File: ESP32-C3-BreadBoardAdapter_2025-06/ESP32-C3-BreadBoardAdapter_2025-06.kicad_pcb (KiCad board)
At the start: 2 copper layers, 52.1 x 40.6 mm, 32 parts, among them J1 PWR, J2 USB-C_Receptacle_Data_16P_GCT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, J3 PWR_JMP, J4 PWR_JMP, J6 Debug_3V3, SW1 SW_Push_SMD_6x3.5, SW2 SW_Push_SMD_6x3.5, SW3 SW_Push_SMD_6x3.5, U1 ESP32-C3-WROOM-02-N4, U2 AMS1117-3V3, U3 L7805

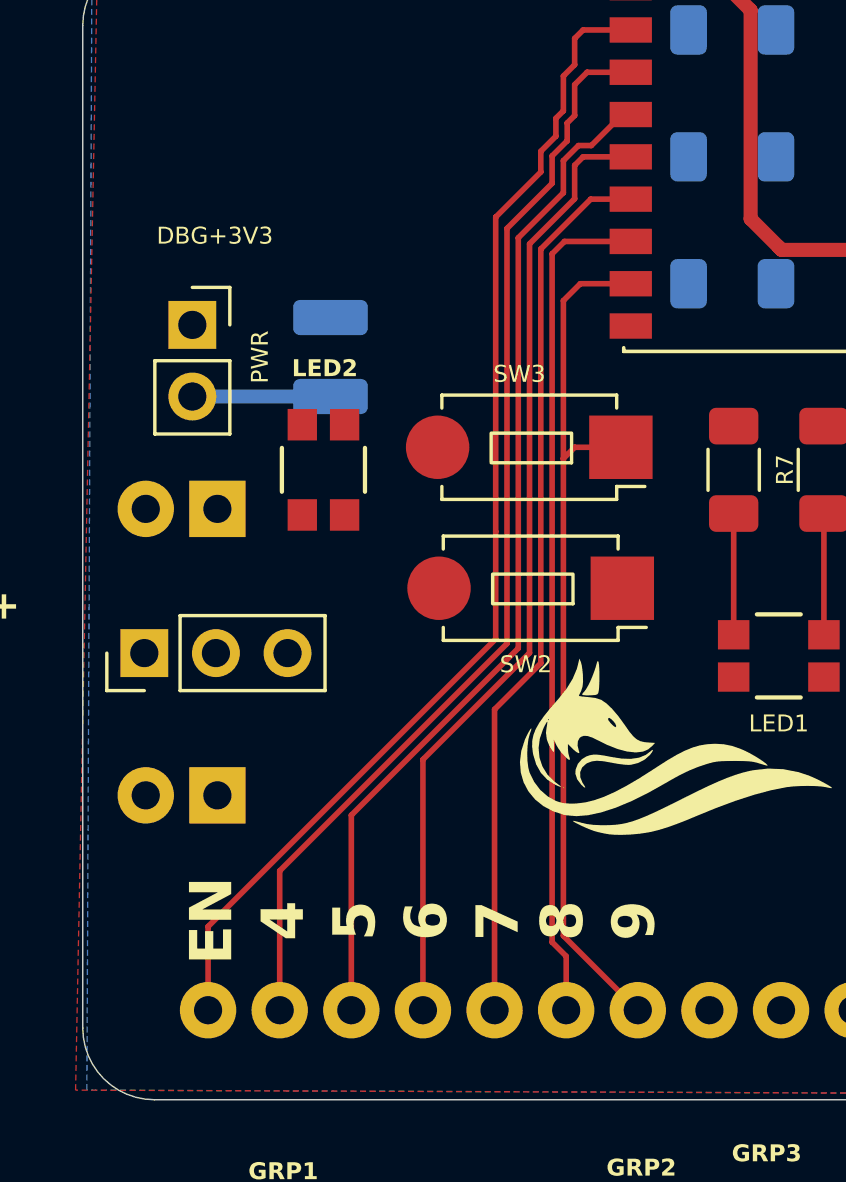
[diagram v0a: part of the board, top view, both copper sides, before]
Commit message: .
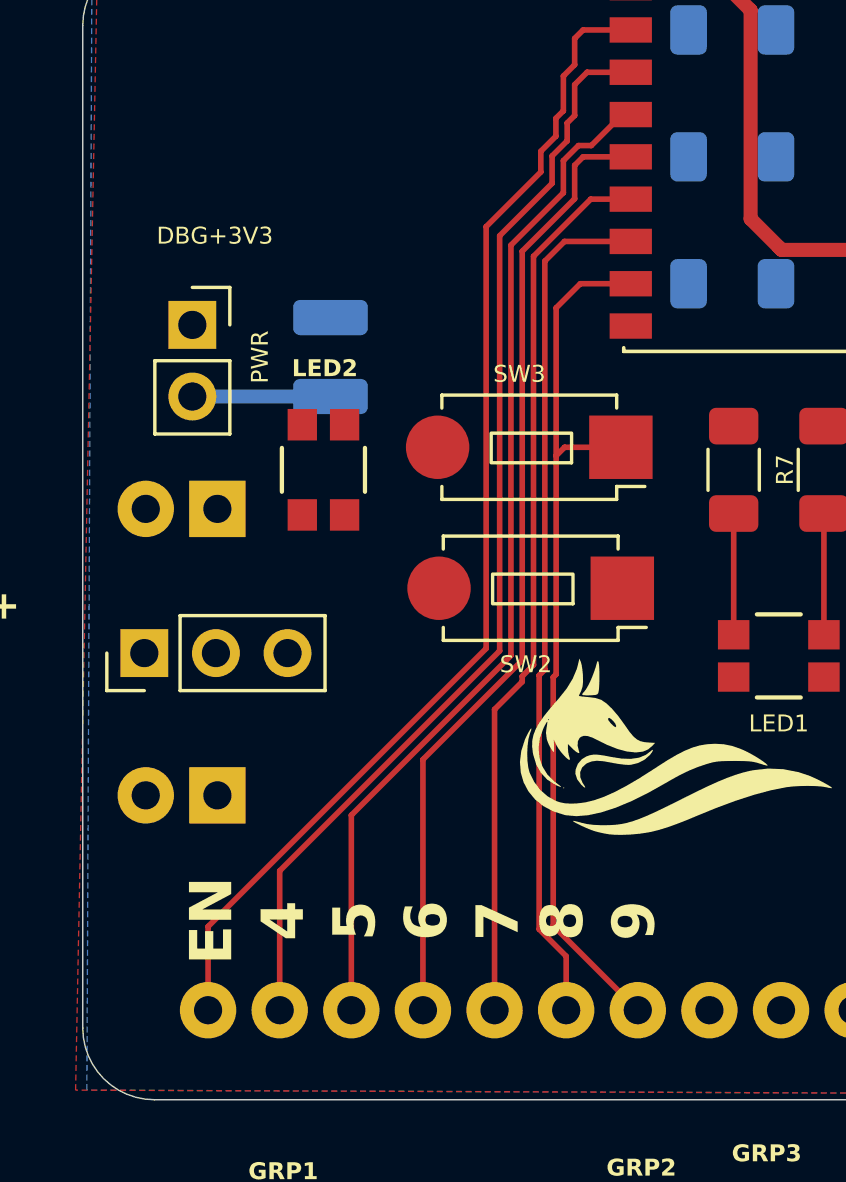
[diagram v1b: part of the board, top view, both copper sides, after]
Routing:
- net /IO9: track 31.1 -> 31.6 mm
